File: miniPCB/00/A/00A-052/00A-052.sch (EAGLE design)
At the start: 7 parts

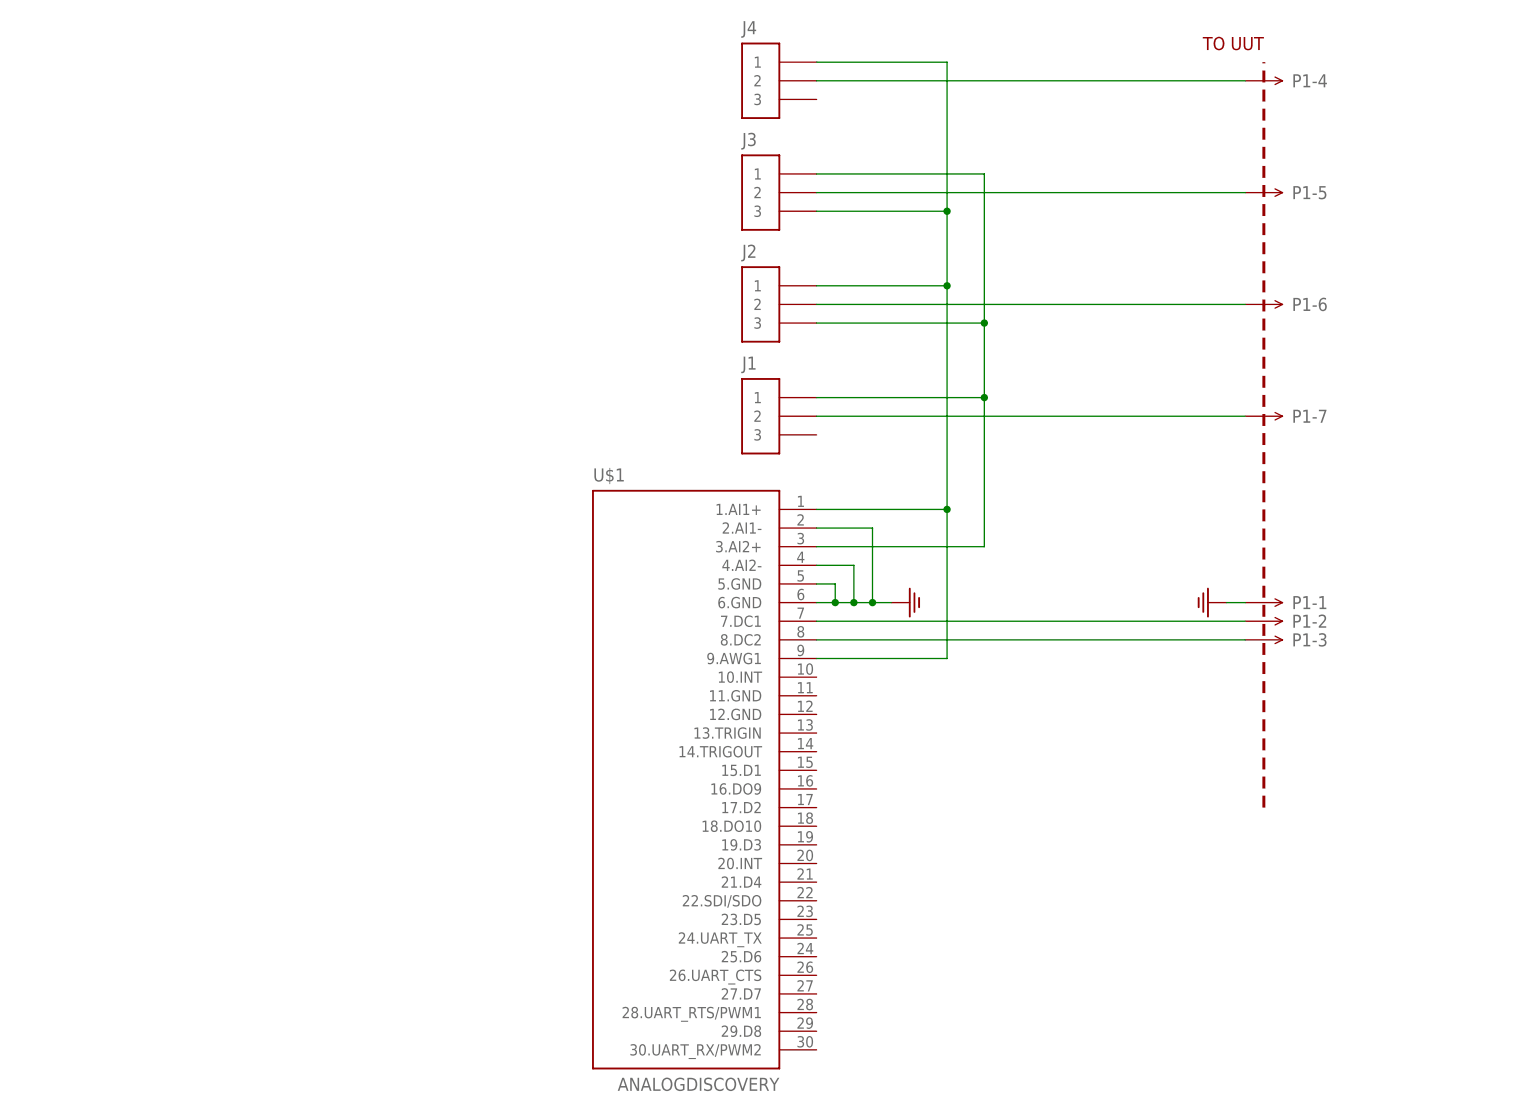
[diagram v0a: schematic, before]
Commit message: Attempting to fix my Git merge error.
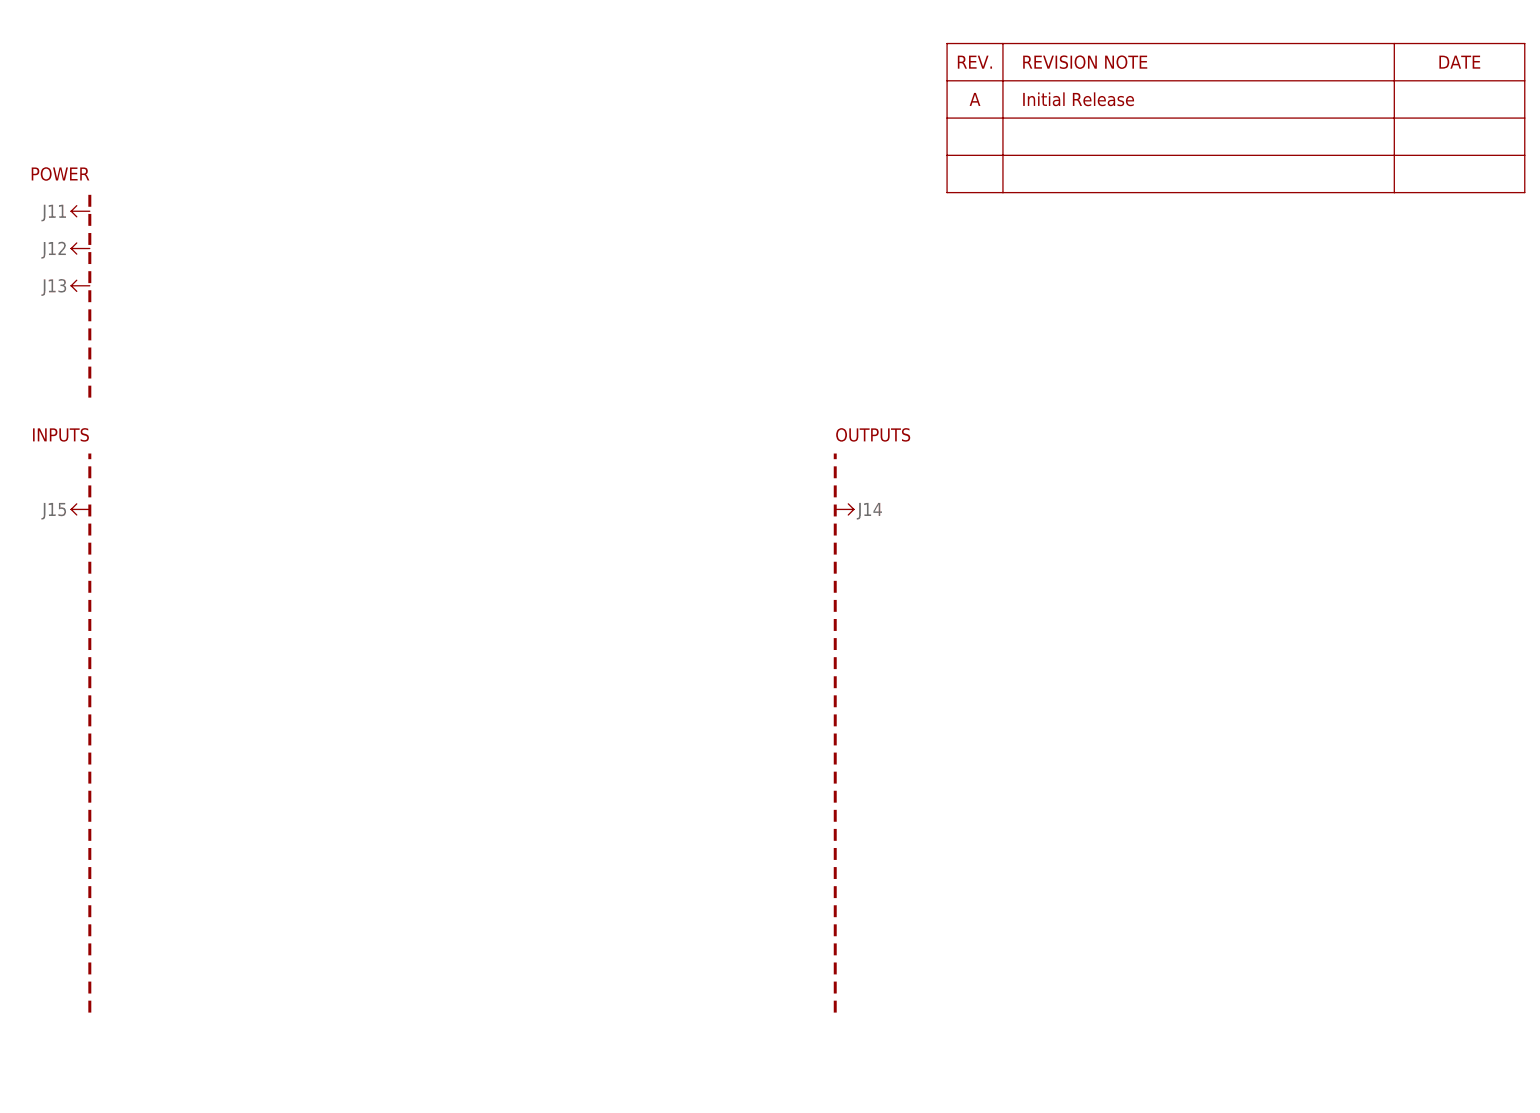
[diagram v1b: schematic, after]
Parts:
- removed J2, J3, J4: (no value), minipcb:PINS_3_2.54
- removed P1: (no value), minipcb:MINIPCB_7P
- removed PCB1: TO UUT, minipcb:MINIPCB_0P25X50
- removed U$1: ANALOGDISCOVERY, minipcb:ANALOGDISCOVERY
- J1: device minipcb:PINS_3_2.54 -> minipcb:MINIPCB_5P20X15
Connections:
- removed net GND: P1-1.1, U$1.2.AI1-, U$1.4.AI2-, U$1.5.GND, U$1.6.GND
- removed net N$1: P1-2.1, U$1.7.DC1
- removed net N$10: J1.1, J2.3, J3.1, U$1.3.AI2+
- removed net N$11: J2.1, J3.3, J4.1, U$1.1.AI1+, U$1.9.AWG1
- removed net N$2: P1-3.1, U$1.8.DC2
- removed net N$3: J1.2, P1-7.1
- removed net N$4: J2.2, P1-6.1
- removed net N$7: J3.2, P1-5.1
- removed net N$8: J4.2, P1-4.1
